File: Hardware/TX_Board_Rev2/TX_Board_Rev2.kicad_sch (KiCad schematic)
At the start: 41 parts, among them IC1 GP2Y1+, IC2 GP2Y1+, IC24 ADP5600ACPZ-R7, IC25 TPS7A4701RGWT, IC27 ADPL40502AUJZ-1.8-R7, IC3 GP2Y1+, J1 Conn_Coaxial, J10 MM8030-2610RJ3, J11 MM8030-2610RJ3, J12 MM8030-2610RJ3, J19 694106301002, J20 Conn_01x08, J9 MM8030-2610RJ3, U1 SN74HCT138NSR

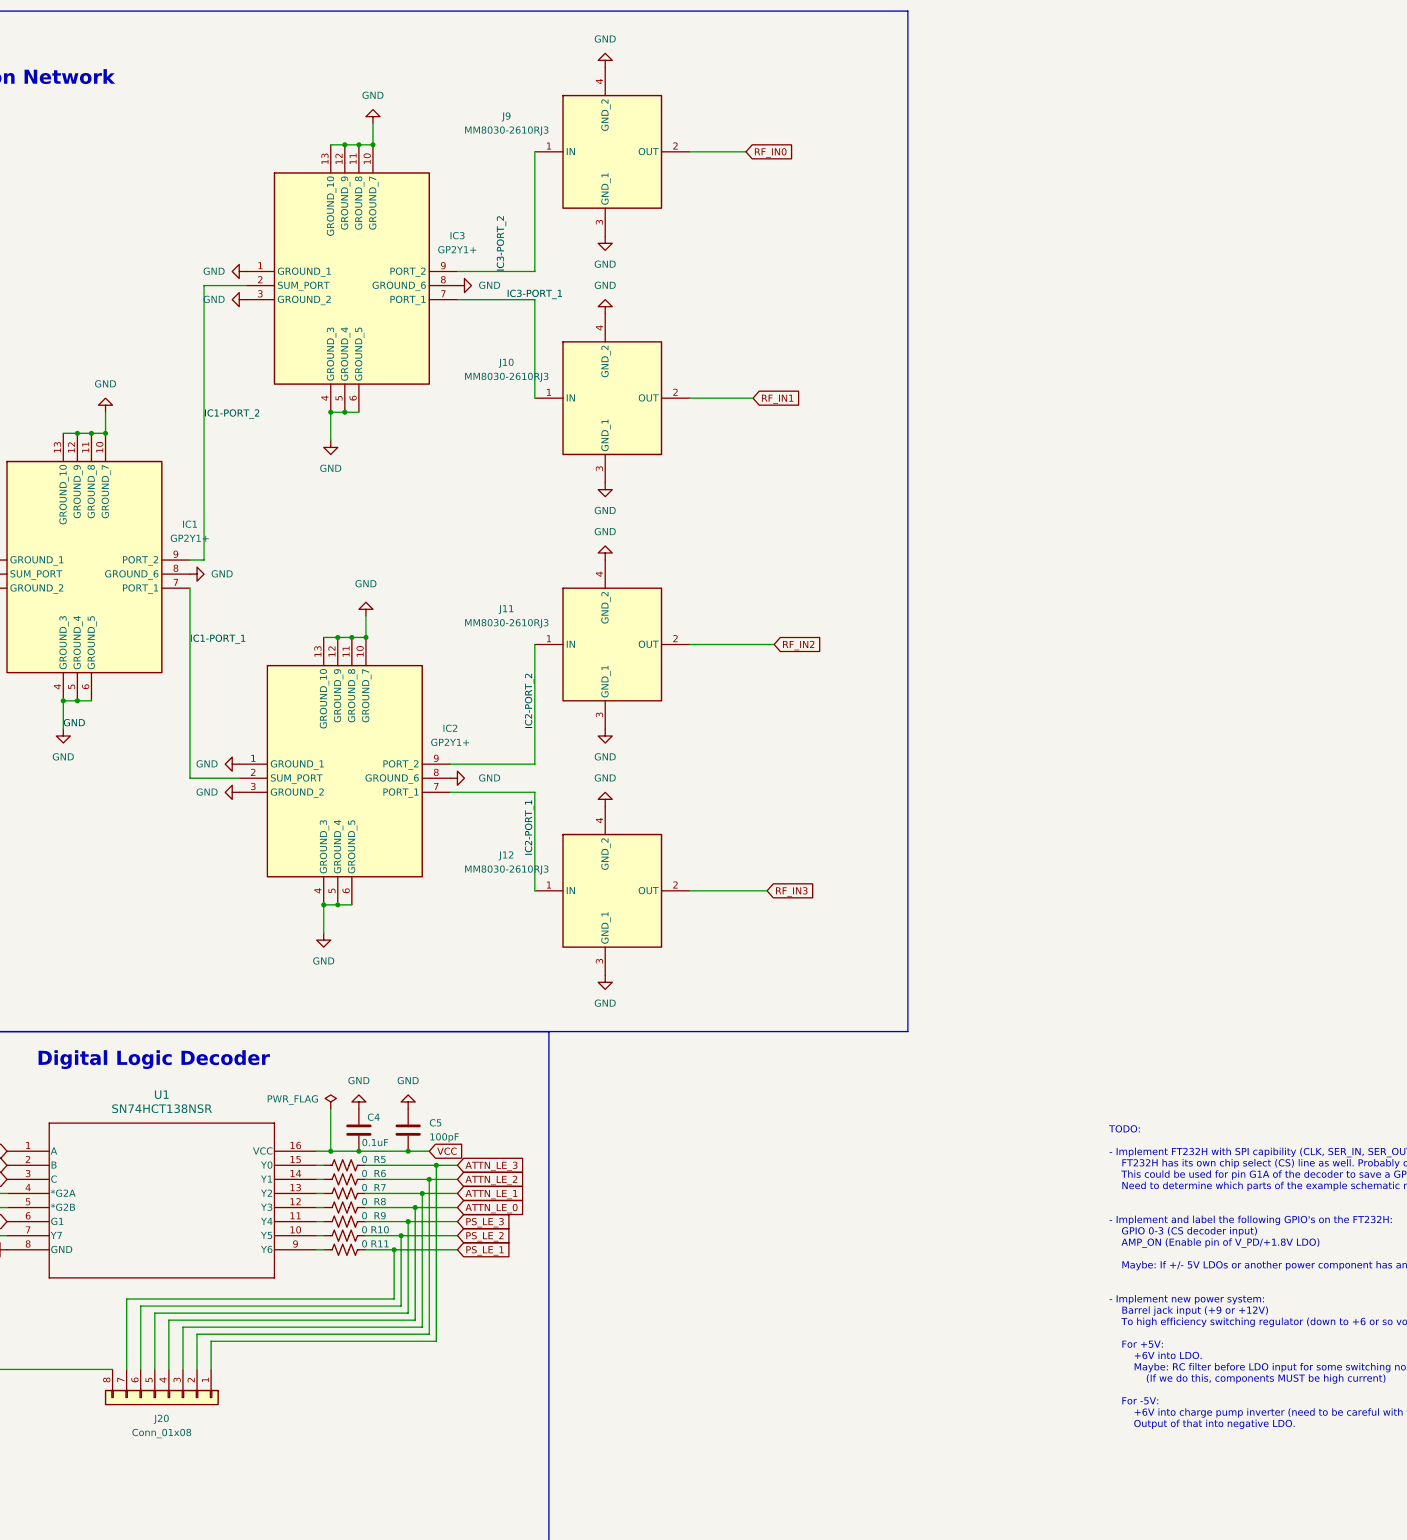
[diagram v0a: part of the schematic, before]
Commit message: Rev2 Progress
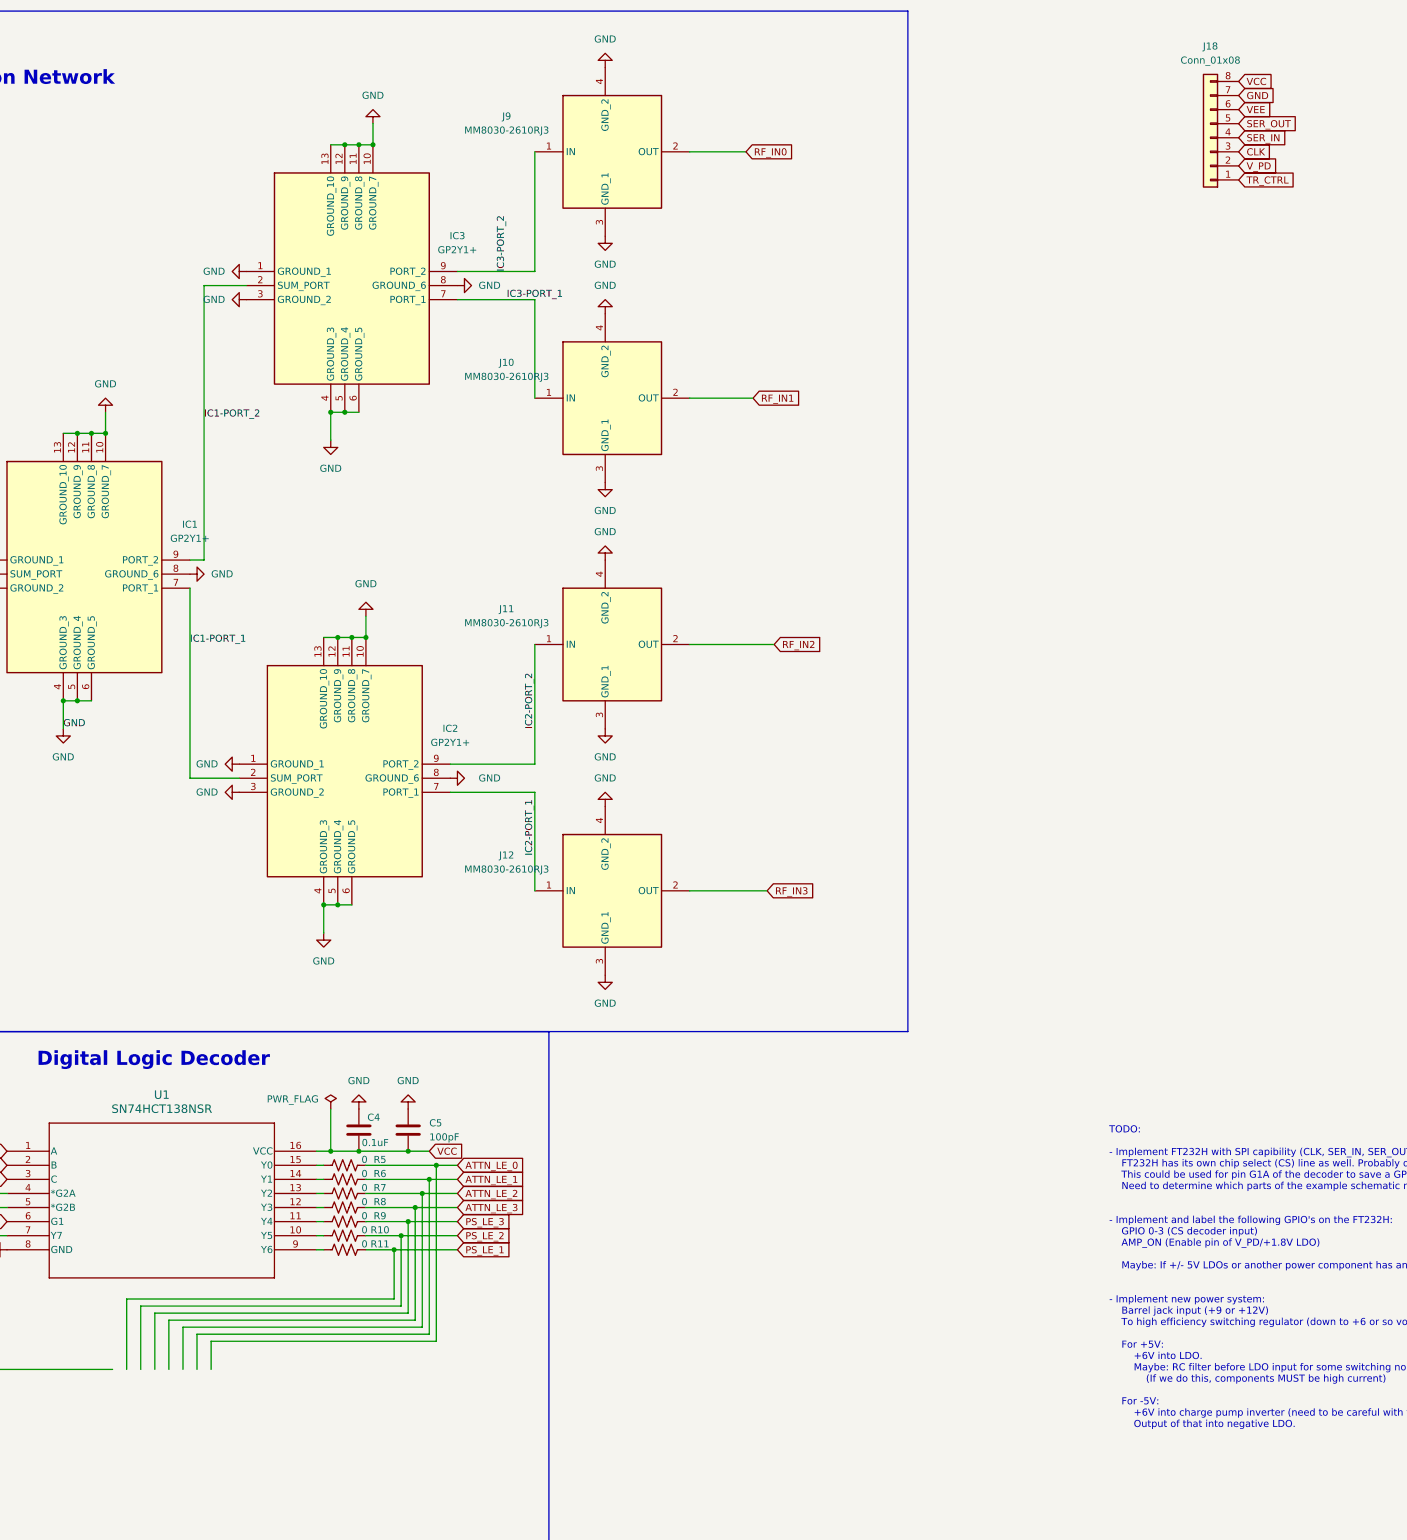
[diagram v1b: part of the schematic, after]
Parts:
- removed J20: Conn_01x08, Connector_PinHeader_2.54mm:PinHeader_1x08_P2.54mm_Horizontal, symbol Connector_Generic:Conn_01x08
- added J18: Conn_01x08, Connector_PinHeader_2.54mm:PinHeader_1x08_P2.54mm_Vertical, symbol Connector_Generic:Conn_01x08
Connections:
- net ATTN_LE_0: now also R5.2; no longer R8.2
- net ATTN_LE_1: now also R6.2; no longer R7.2
- net ATTN_LE_2: now also R7.2; no longer R6.2
- net ATTN_LE_3: now also R8.2; no longer R5.2
- net CLK: now also J18.3 (Pin_3)
- net GND: now also J18.7 (Pin_7)
- net SER_IN: now also J18.4 (Pin_4)
- net SER_OUT: now also J18.5 (Pin_5)
- net TR_CTRL: now also J18.1 (Pin_1)
- net VCC: now also J18.8 (Pin_8)
- net VEE: now also J18.6 (Pin_6)
- net V_PD: now also J18.2 (Pin_2)
